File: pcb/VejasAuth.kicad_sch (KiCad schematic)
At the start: 37 parts, among them J1 USB_A, J3 UP20-C-F-G-FL-P12-TR, SW1 PTS815 SJM 250 SMTR LFS, SW2 PTS815 SJM 250 SMTR LFS, U2 W25Q128JVS, U3 XC6206P332MR-G, U4 RP2350A-QFN60, Y1 ABM8-272-T3

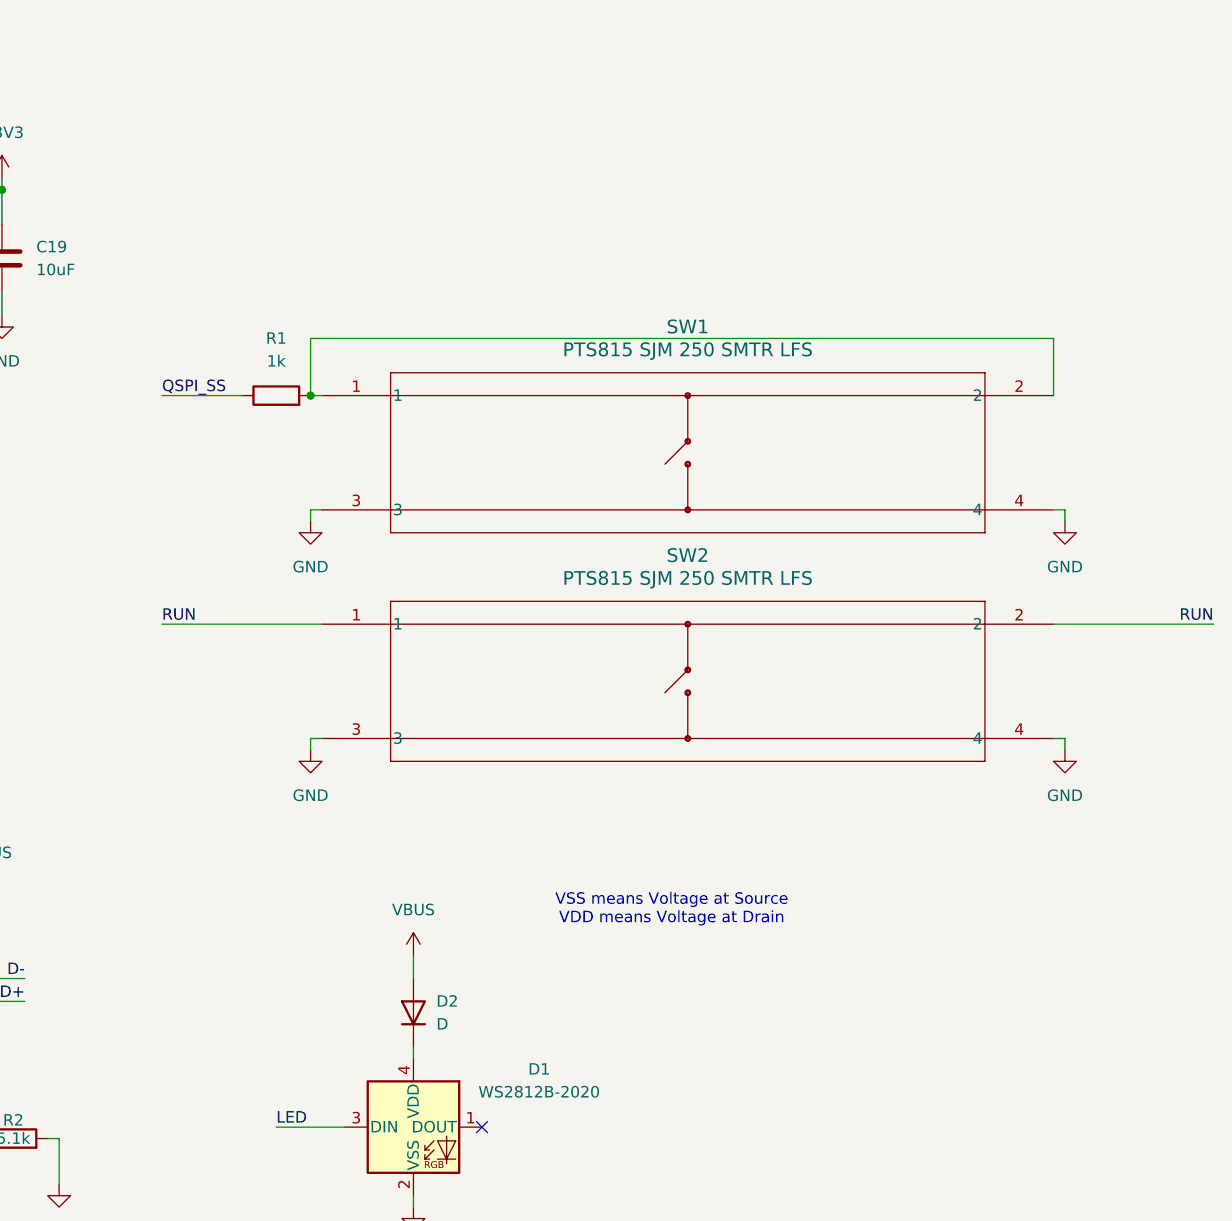
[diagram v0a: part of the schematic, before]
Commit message: cool stuff V1 i think
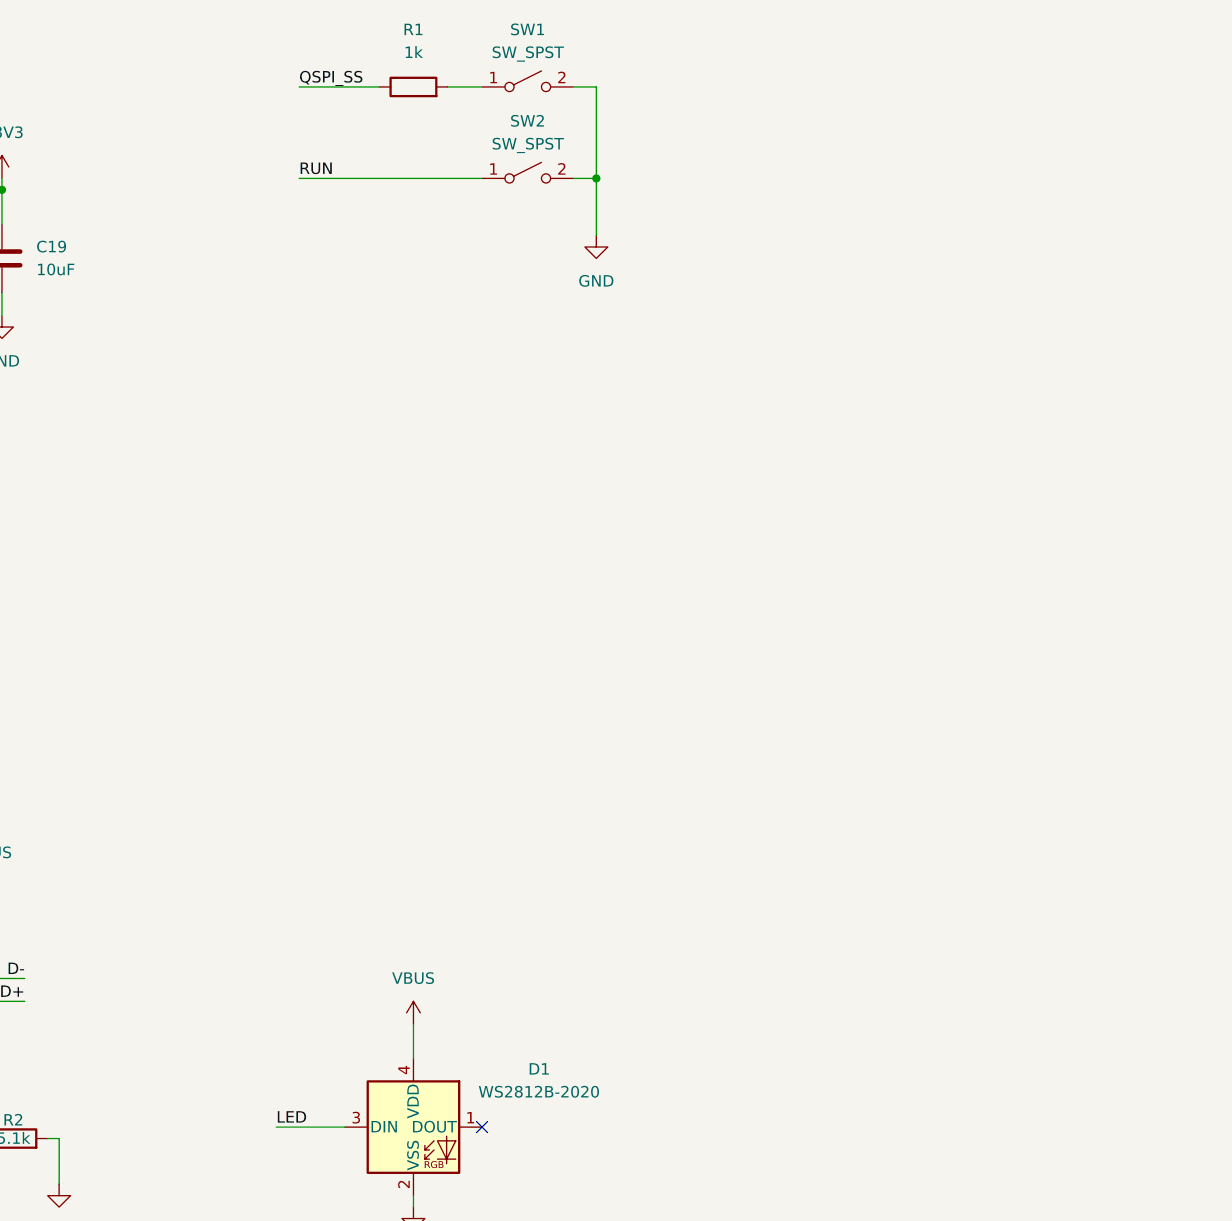
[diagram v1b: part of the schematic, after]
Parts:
- removed D2: D, Diode_SMD:D_0402_1005Metric, symbol Device:D
- removed SW1, SW2: PTS815 SJM 250 SMTR LFS, PTS815SJM250SMTRLFS:SW4_PTS815 SJM 250 SMTR LFS_CNK, symbol PTS815SJM250SMTRLFS:PTS815_SJM_250_SMTR_LFS
- added SW1, SW2: SW_SPST, Button_Switch_SMD:SW_Push_SPST_NO_Alps_SKRK, symbol Switch:SW_SPST
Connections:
- net GND: now also SW1.2 (B), SW2.2 (B)
- net RUN: now also SW2.1 (A)
- net VBUS: now also D1.4 (VDD)
- net at R1.2: now also SW1.1 (A)
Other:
- note removed: "VSS means Voltage at Source VDD means Voltage at Drain"
- moved on the sheet: R1

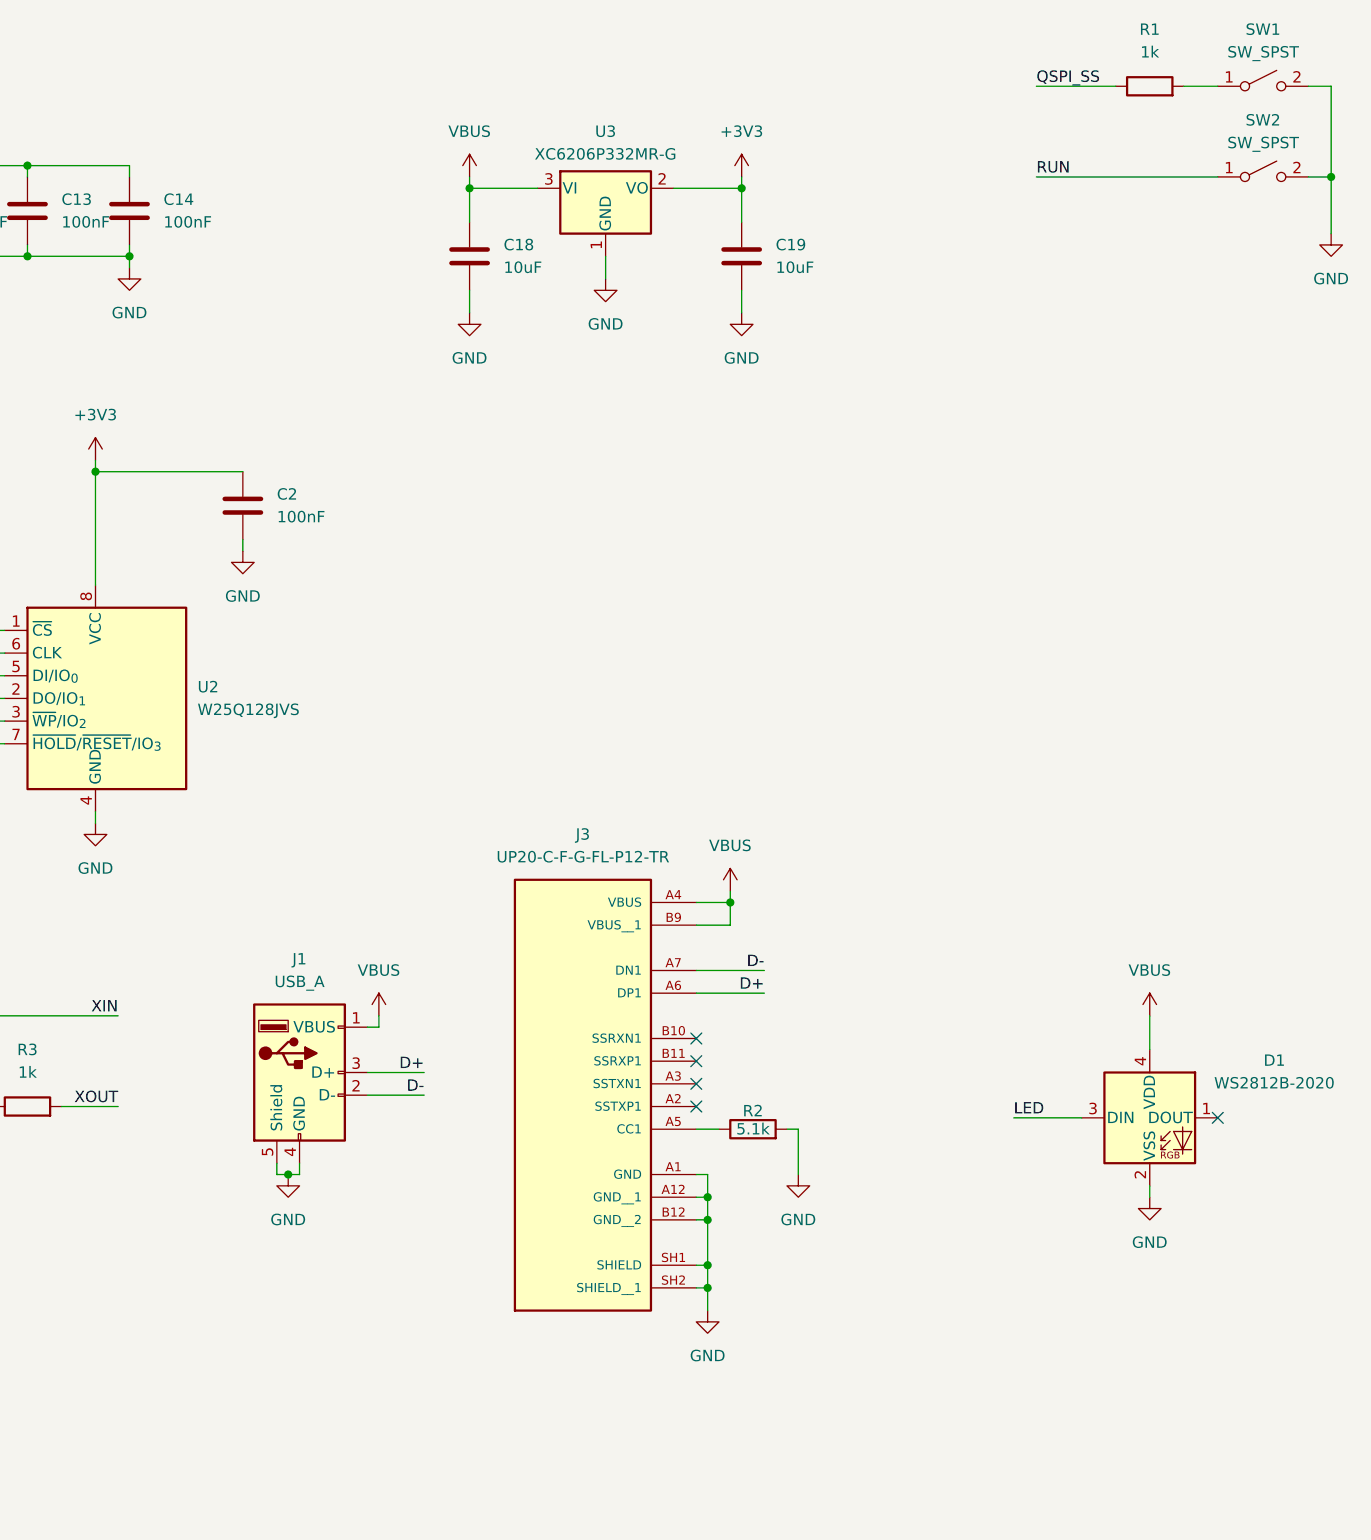
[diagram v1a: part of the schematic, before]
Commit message: big update
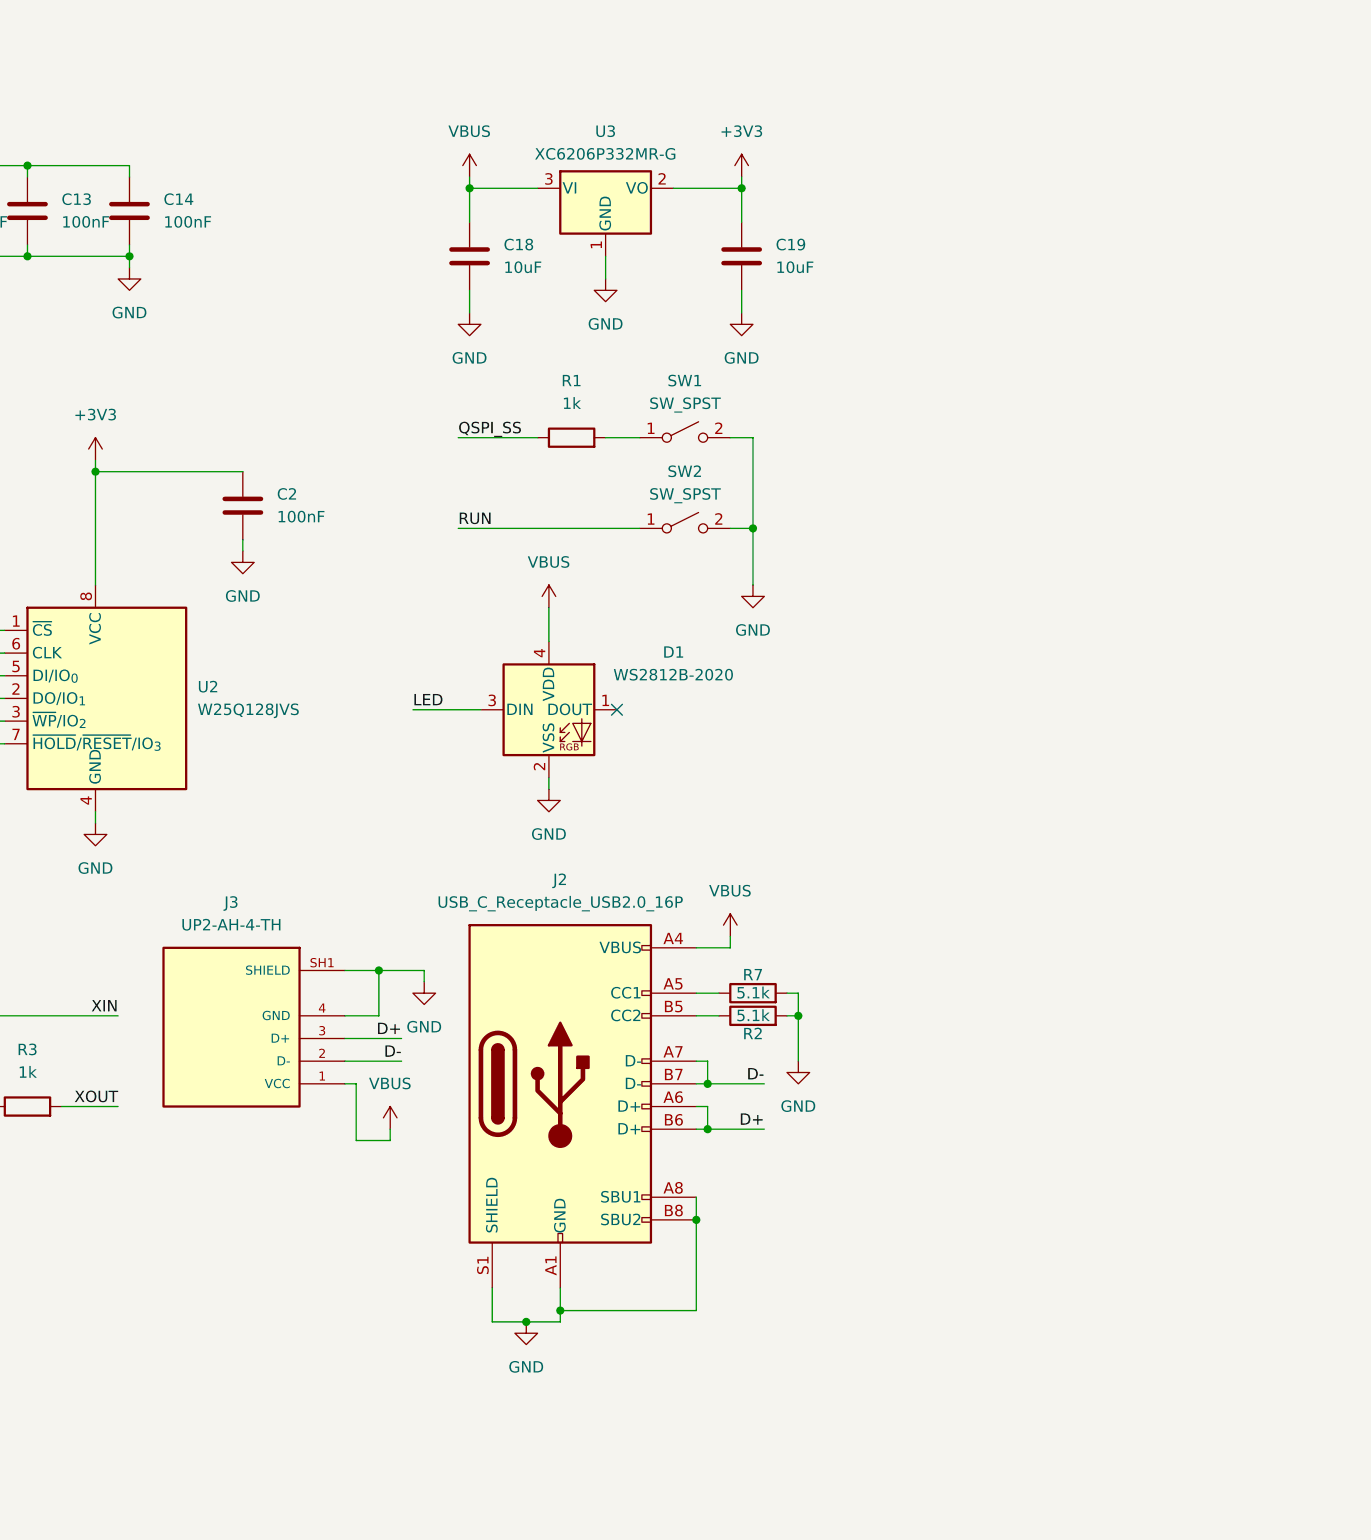
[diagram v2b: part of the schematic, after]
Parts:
- removed J1: USB_A, Connector_USB:USB_A_Molex_48037-2200_Horizontal, symbol Connector:USB_A
- removed J3: UP20-C-F-G-FL-P12-TR, footprint:SAMESKY_UP20-C-F-G-FL-P12-TR, symbol usbc:UP20-C-F-G-FL-P12-TR
- added J2: USB_C_Receptacle_USB2.0_16P, Connector_USB:USB_C_Receptacle_GCT_USB4105-xx-A_16P_TopMnt_Horizontal, symbol Connector:USB_C_Receptacle_USB2.0_16P
- added J3: UP2-AH-4-TH, usb a tht:CUI_UP2-AH-4-TH, symbol usb a tht:UP2-AH-4-TH
- added R7: 5.1k, Resistor_SMD:R_0402_1005Metric, symbol Device:R
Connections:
- net D+: now also J2.A6 (D+), J2.B6 (D+), J3.3 (D+)
- net D-: now also J2.A7 (D-), J2.B7 (D-), J3.2 (D-)
- net GND: now also J2.A1 (GND), J2.A12 (GND), J2.A8 (SBU1), J2.B1 (GND), J2.B12 (GND), J2.B8 (SBU2), J2.S1 (SHIELD), J3.4 (GND), J3.SH1 (SHIELD), J3.SH2 (SHIELD), R7.2
- net VBUS: now also J2.A4 (VBUS), J2.A9 (VBUS), J2.B4 (VBUS), J2.B9 (VBUS), J3.1 (VCC)
- net at R2.1: now also J2.B5 (CC2)
- new net: J2.A5 (CC1), R7.1
- no-connect marks 5 -> 1
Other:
- moved on the sheet: D1, R1, R2, SW1, SW2
